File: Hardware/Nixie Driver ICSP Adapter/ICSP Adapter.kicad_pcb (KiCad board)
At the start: 2 copper layers, 24.1 x 33.7 mm, 5 parts

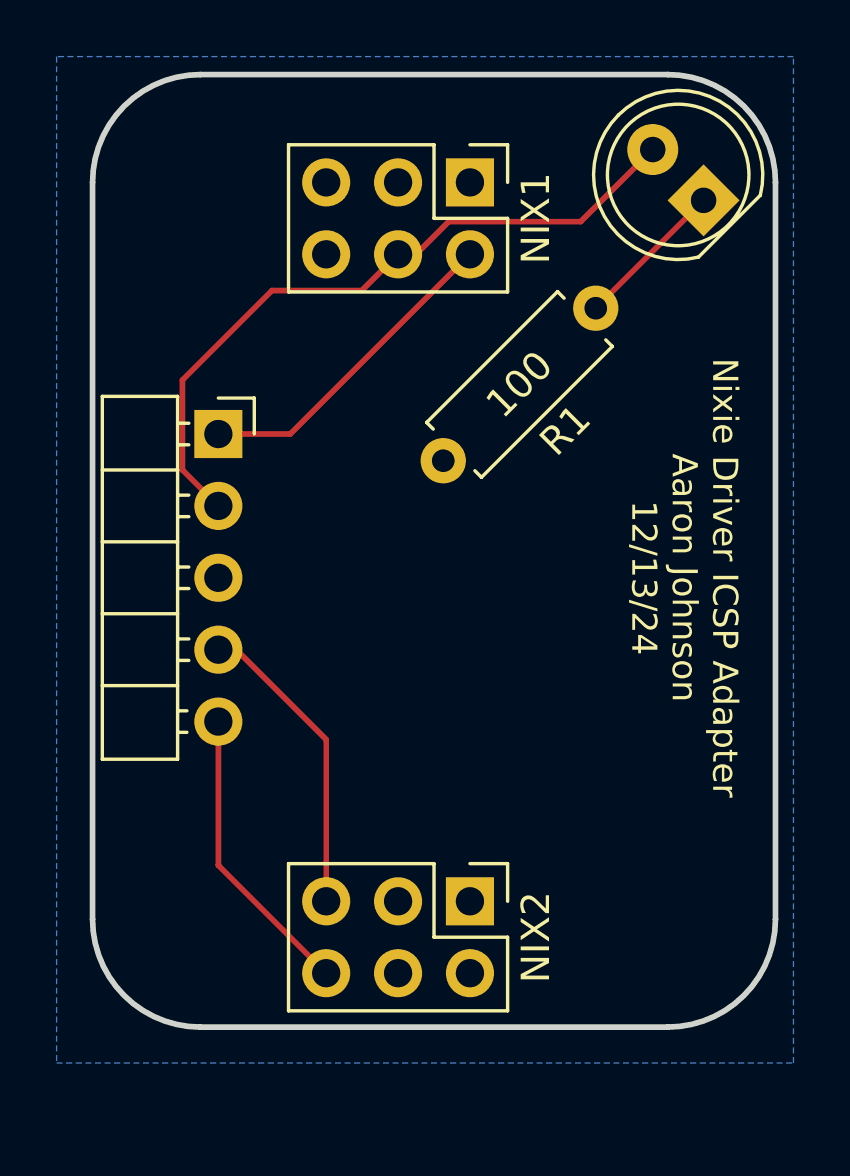
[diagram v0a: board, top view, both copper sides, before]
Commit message: V2 ICSP adapter
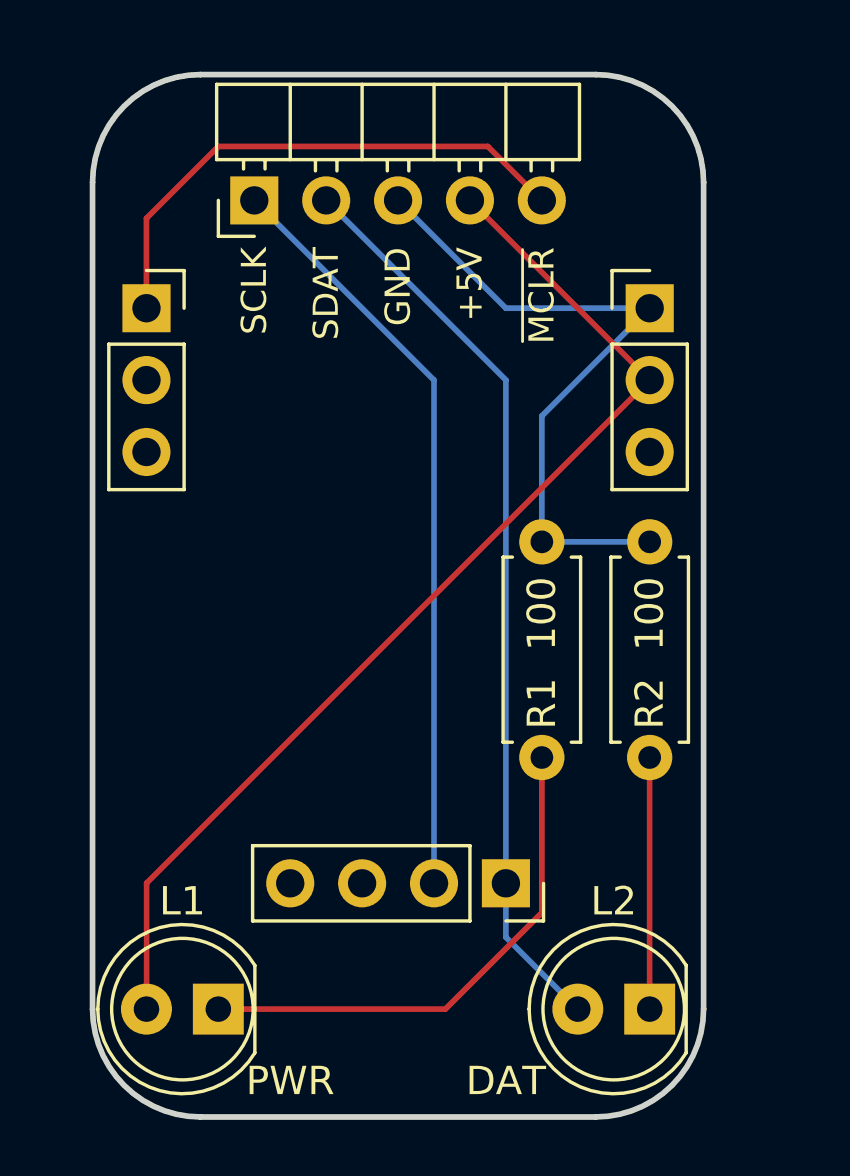
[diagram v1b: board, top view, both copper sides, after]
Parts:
- removed NIX1, NIX2: HDRF-2X3, Connector_PinHeader_2.54mm:PinHeader_2x03_P2.54mm_Vertical
- added L2: DAT, LED_THT:LED_D5.0mm, F.Cu at (135.9, 142.2)
- added N1: ~, Nixie:Nixie Driver V2, F.Cu at (127.0, 125.1)
- added R2: 100, Resistor_THT:R_Axial_DIN0207_L6.3mm_D2.5mm_P7.62mm_Horizontal, F.Cu at (135.9, 133.3)
- J1: renamed from ICSP0; value HDR-1X5H -> ICSP
- L1: renamed from PWR0; value LED-5MM_ROUND_GREEN -> PWR
- moved L1 33.3 mm to (120.7, 142.2), turned to 180 degrees
- moved J1 18.5 mm to (121.9, 113.7), turned to 90 degrees
- moved R1 16.0 mm to (132.1, 133.3), turned to 90 degrees
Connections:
- net LED renamed Net-(L1-K)
- J1 pad 1: ~{MCLR} -> SCLK
- J1 pad 2: VDD -> SDAT
- J1 pad 4: SDAT -> VDD
- J1 pad 5: SCLK -> ~{MCLR}
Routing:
- net GND: track 0.00 -> 24.1 mm
- net SDAT: track 10.8 -> 32.3 mm
- net SCLK: track 10.5 -> 26.8 mm
- net VDD: track 25.0 -> 38.6 mm
- net Net-(L1-K): track 5.39 -> 18.3 mm
- net Net-(L2-K): track 0.00 -> 8.89 mm
- net ~{MCLR}: track 11.5 -> 19.0 mm
- removed copper zone on B.Cu, net GND
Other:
- board size 24.1 x 33.7 mm -> 21.6 x 36.8 mm
- board text added: "Nixie Driver V2 ICSP Adapter Aaron Johnson 02/05/2025"
- board text removed: "Nixie Driver ICSP Adapter Aaron Johnson 12/13/24"
